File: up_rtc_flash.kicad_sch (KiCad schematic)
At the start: 1 part

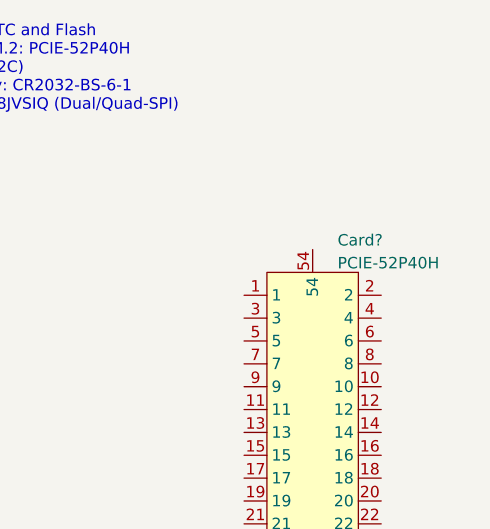
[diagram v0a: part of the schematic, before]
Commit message: updated library, partly created power.kicad_sch
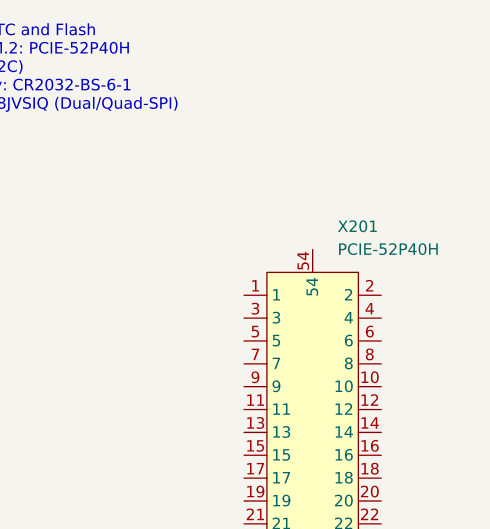
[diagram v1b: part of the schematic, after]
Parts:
- gave numbers to parts that had none: 1
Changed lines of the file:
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@@
   (symbol (lib_id "eduboardv2:PCIE-52P40H") (at 63.5 77.47 270) (unit 1)
     (in_bom yes) (on_board yes) (fields_autoplaced)
-    (property "Reference" "Card?" (id 0) (at 66.2687 38.3372 90)
+    (property "Reference" "X201" (id 0) (at 66.2687 36.83 90)
       (effects (font (size 1.27 1.27)) (justify left))
     )
-    (property "Value" "PCIE-52P40H" (id 1) (at 66.2687 40.8741 90)
+    (property "Value" "PCIE-52P40H" (id 1) (at 66.2687 39.37 90)
       (effects (font (size 1.27 1.27)) (justify left))
     )
